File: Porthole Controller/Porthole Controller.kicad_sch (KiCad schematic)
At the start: 19 parts, among them J1 Conn_02x03_Counter_Clockwise, J2 Conn_01x03, J3 Screw_Terminal_01x03, J4 Screw_Terminal_01x03, J5 Screw_Terminal_01x03, J6 Screw_Terminal_01x03, J7 Screw_Terminal_01x02, SW1 SW_Push, U1 113991054, U2 SN74AHCT125DR

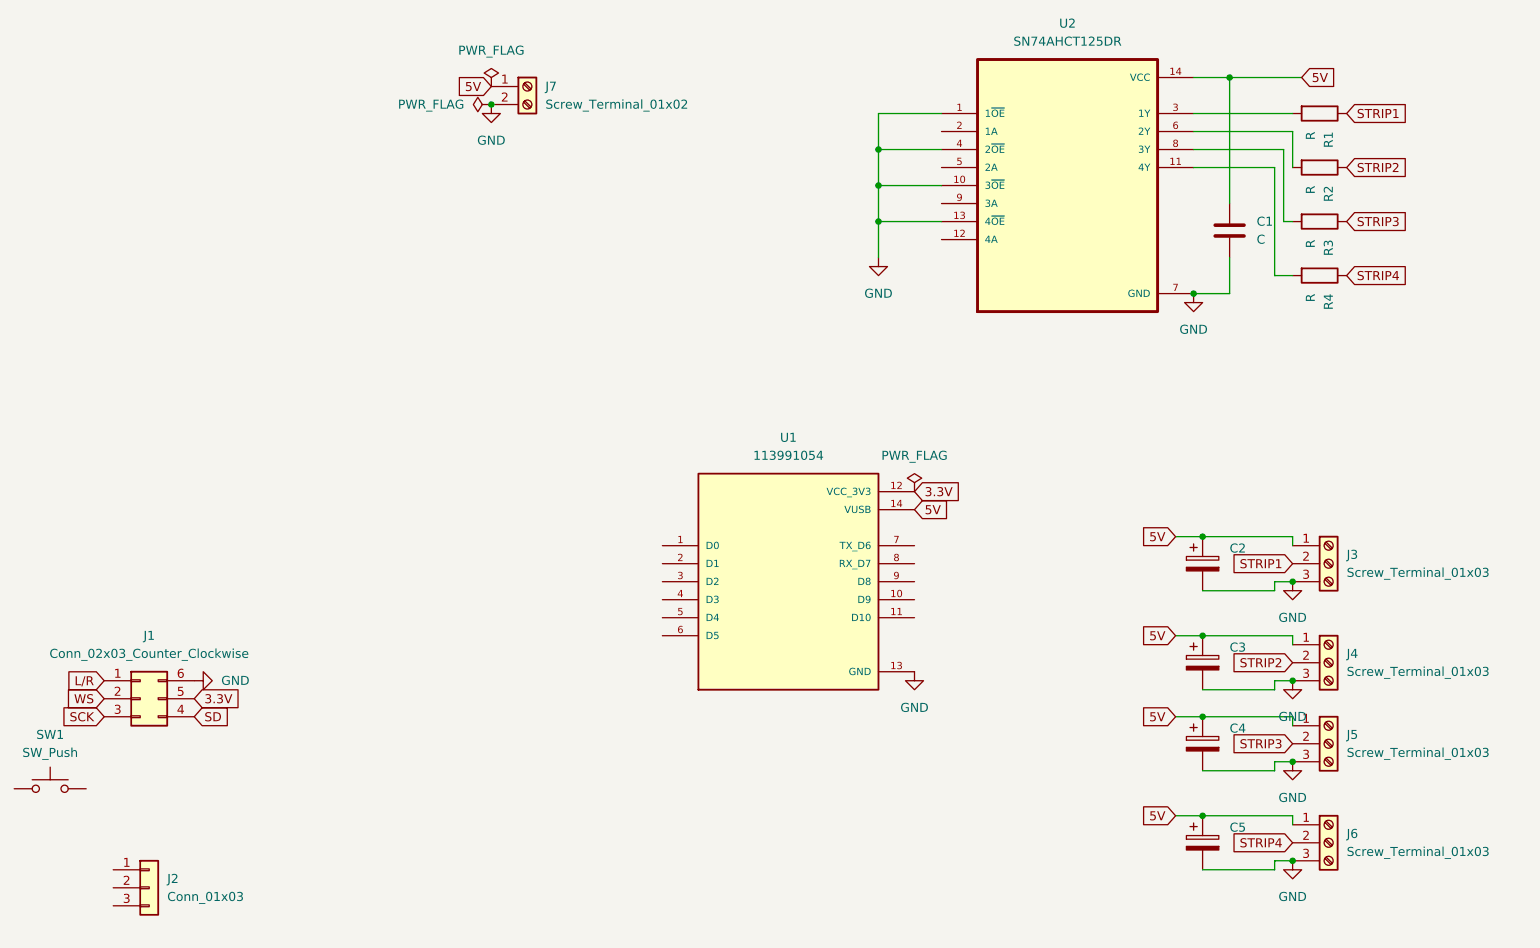
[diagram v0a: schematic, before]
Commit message: Completed schematic
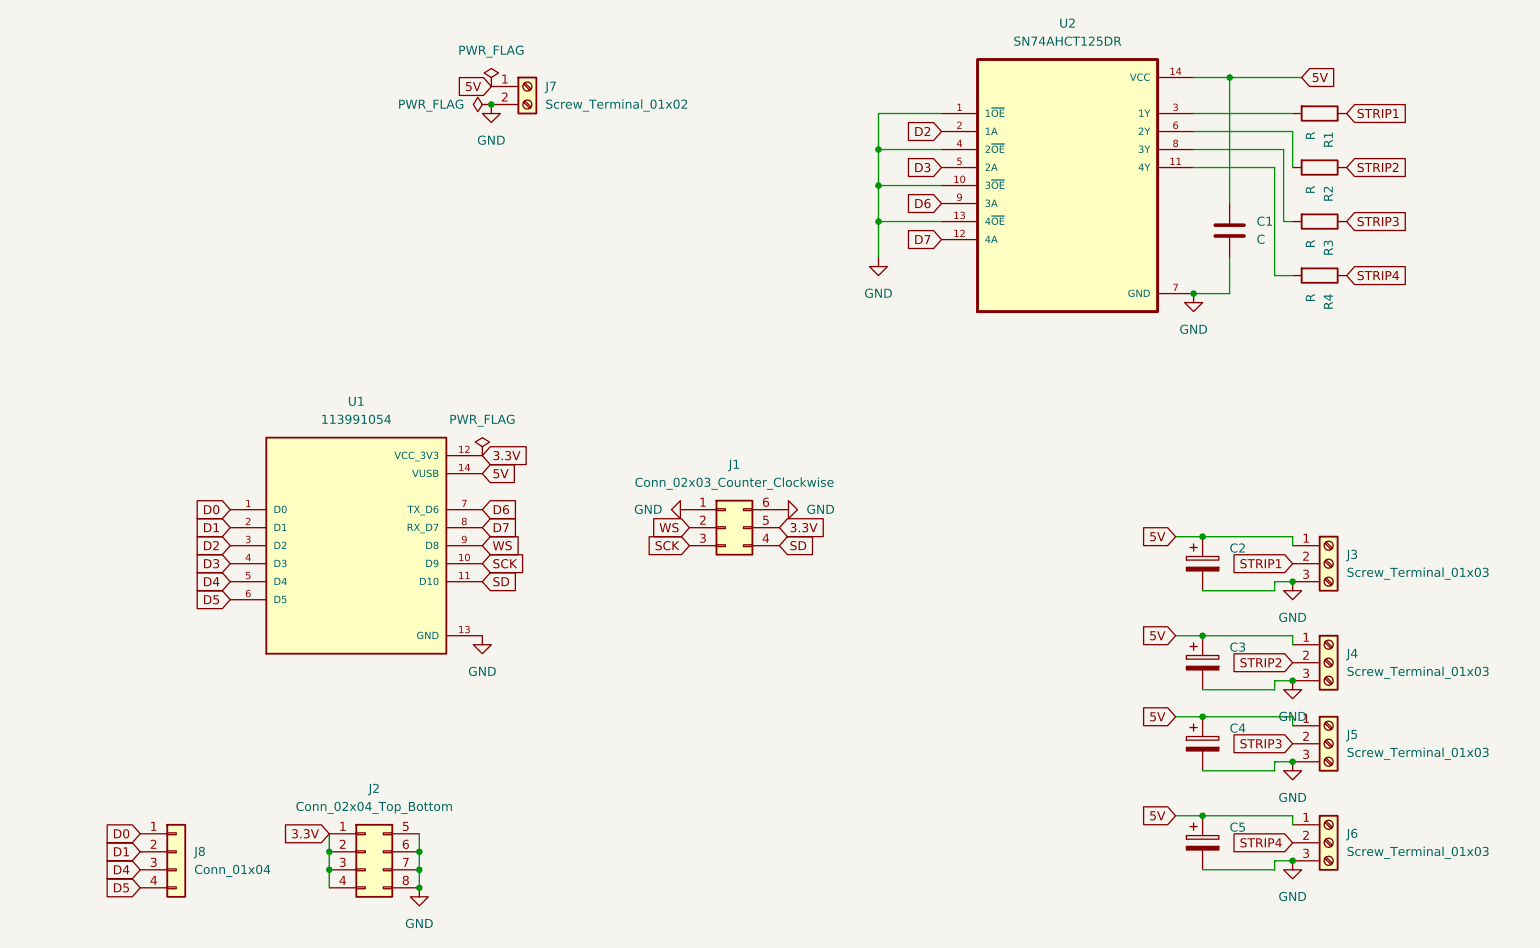
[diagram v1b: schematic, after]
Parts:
- removed J2: Conn_01x03, symbol Connector_Generic:Conn_01x03
- removed SW1: SW_Push, symbol Switch:SW_Push
- added J2: Conn_02x04_Top_Bottom, symbol Connector_Generic:Conn_02x04_Top_Bottom
- added J8: Conn_01x04, symbol Connector_Generic:Conn_01x04
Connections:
- net L/R is gone; now on net GND: J1.1 (Pin_1)
- net 3.3V: now also J2.1 (Pin_1), J2.2 (Pin_2), J2.3 (Pin_3), J2.4 (Pin_4)
- net GND: now also J2.5 (Pin_5), J2.6 (Pin_6), J2.7 (Pin_7), J2.8 (Pin_8)
- net SCK: now also U1.10 (D9)
- net SD: now also U1.11 (D10)
- net WS: now also U1.9 (D8)
- net D0: now reaches U1.1 (D0)
- net D0: now also J8.1 (Pin_1)
- net D1: now reaches U1.2 (D1)
- net D1: now also J8.2 (Pin_2)
- net D2: now reaches U1.3 (D2)
- net D2: now also U2.2 (1A)
- net D3: now reaches U1.4 (D3)
- net D3: now also U2.5 (2A)
- net D4: now reaches U1.5 (D4)
- net D4: now also J8.3 (Pin_3)
- net D5: now reaches U1.6 (D5)
- net D5: now also J8.4 (Pin_4)
- net D6: now reaches U1.7 (TX_D6)
- net D6: now also U2.9 (3A)
- net D7: now reaches U1.8 (RX_D7)
- net D7: now also U2.12 (4A)
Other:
- moved on the sheet: J1, U1
